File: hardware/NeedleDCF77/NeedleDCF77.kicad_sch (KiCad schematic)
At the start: 73 parts, among them J1 USB_C_Receptacle_USB2.0

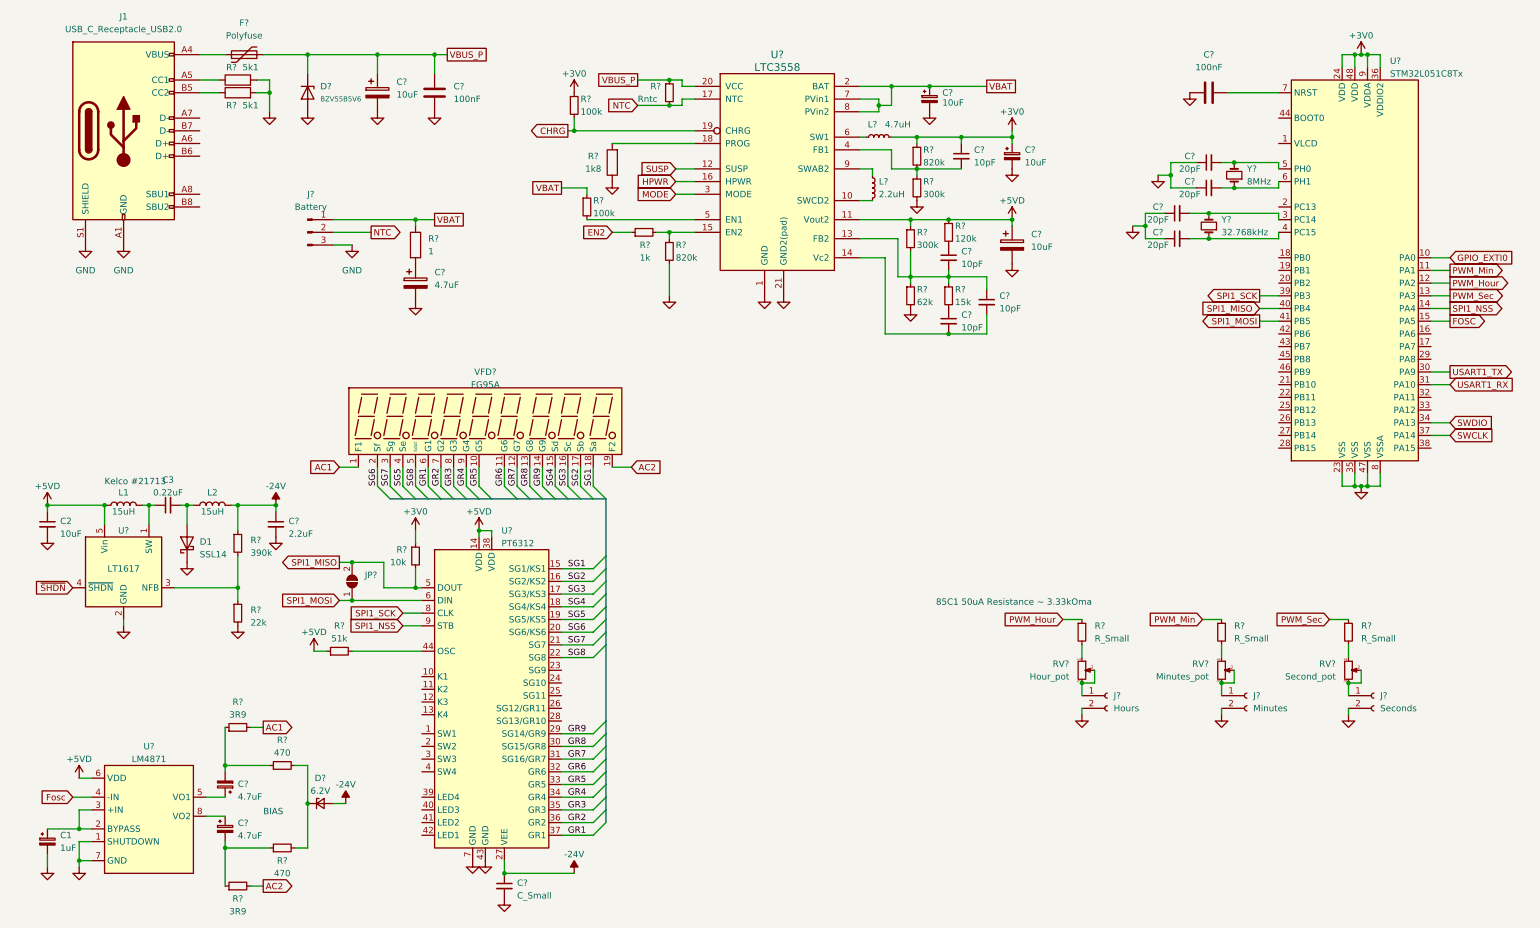
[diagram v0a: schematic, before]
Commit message: Add debug interfaces
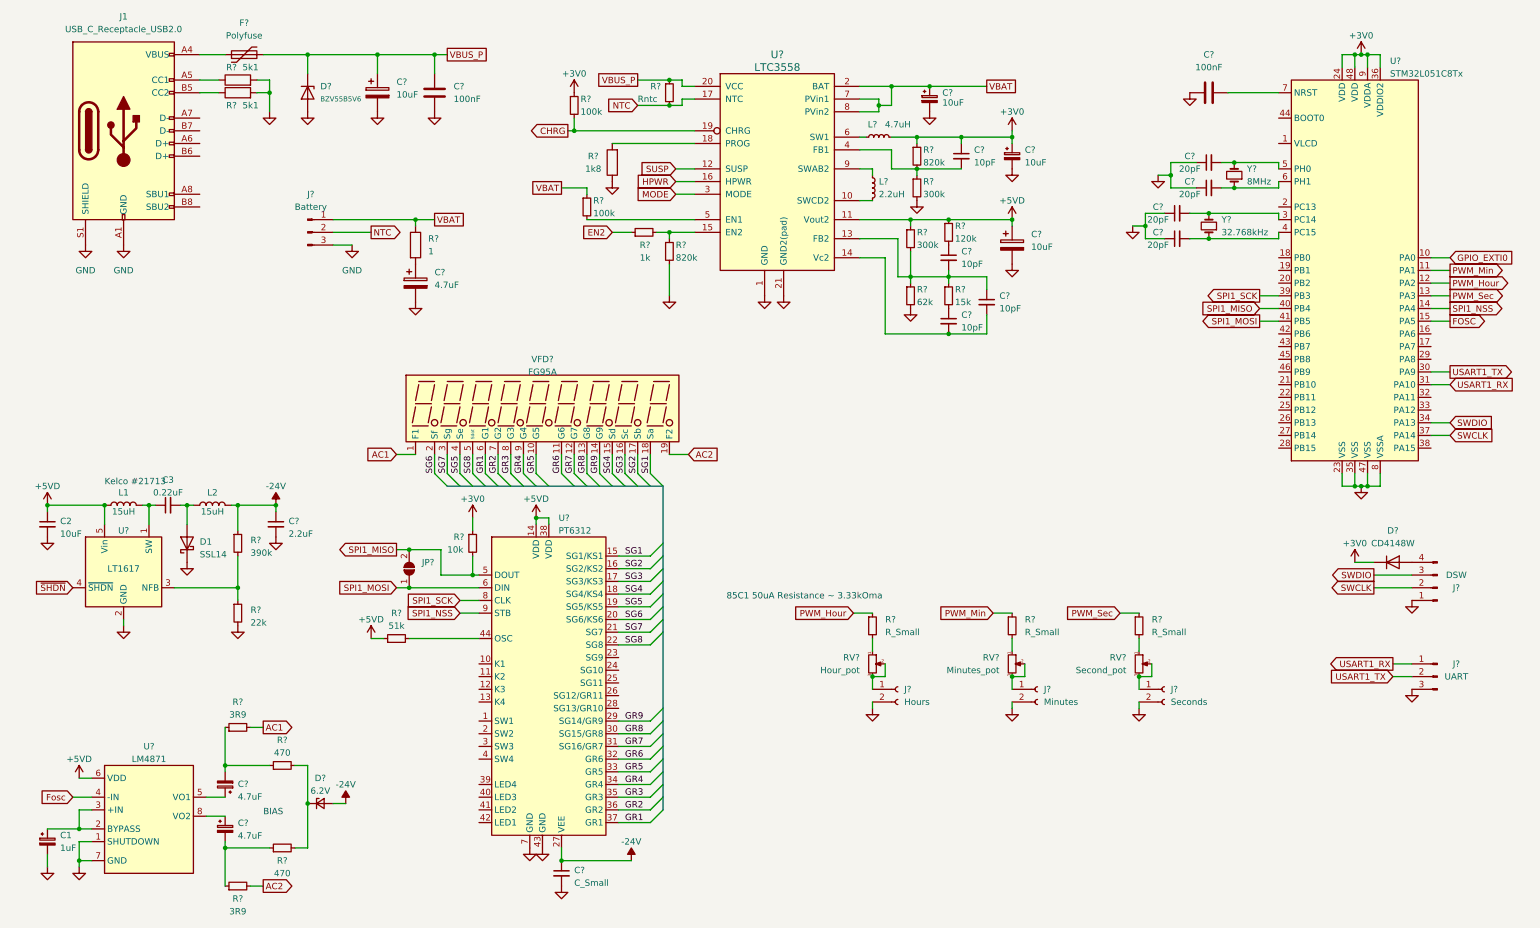
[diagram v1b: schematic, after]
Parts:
- added D?: CD4148W, Diode_SMD:D_0805_2012Metric, symbol Diode:CD4148W
- added J?: UART, symbol Connector:Conn_01x03_Pin
- added J?: DSW, symbol Connector:Conn_01x04_Pin
- JP?: value (none) -> ~
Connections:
- net +3V0: now also D?.1 (K)
- net GND: now also J?.1 (Pin_1), J?.3 (Pin_3)
- net SWCLK: now also J?.2 (Pin_2)
- net SWDIO: now also J?.3 (Pin_3)
- net USART1_RX: now also J?.1 (Pin_1)
- net USART1_TX: now also J?.2 (Pin_2)
- new net: D?.2 (A), J?.4 (Pin_4)
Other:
- moved on the sheet: C?, J?, JP?, R?, RV?, U?, VFD?
